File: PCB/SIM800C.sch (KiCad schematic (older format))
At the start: 35 parts, among them J10 Conn_01x05, J11 Conn_01x02, J8 Conn_01x05, J9 Conn_01x05, U10 GSM_SMA, U11 BT_SMA, U12 USB_PCB, U3 footprint-lib_nano-sim-card-h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, U4 SMF05C, U5 SIM800C, U6 MIC29302BU

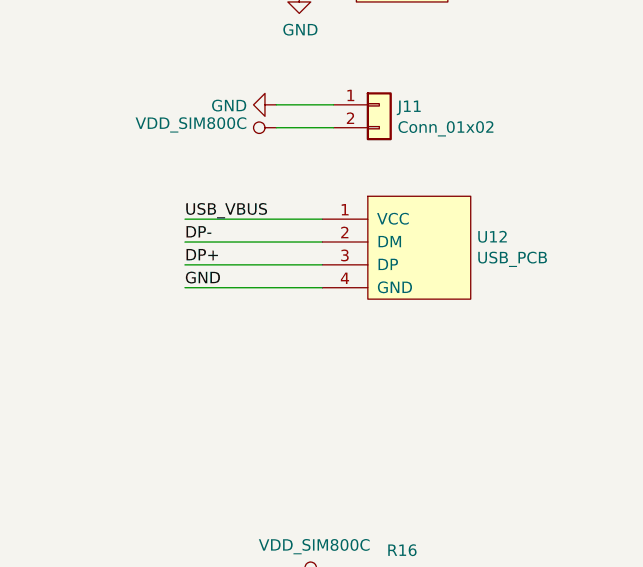
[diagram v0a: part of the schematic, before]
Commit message: updte
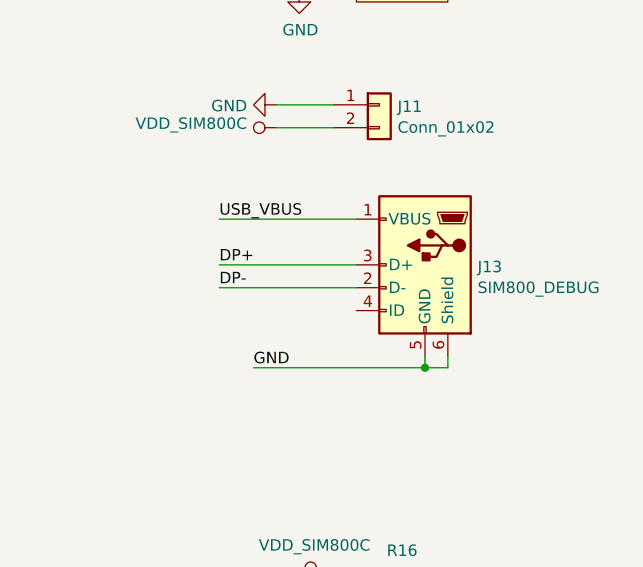
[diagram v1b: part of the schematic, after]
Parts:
- removed U12: USB_PCB, footprint-lib:usb-PCB, symbol taobao-components:USB_PCB
- added J13: SIM800_DEBUG, w_conn_pc:conn_usb_B_micro_smd, symbol Connector:USB_B_Micro
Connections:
- net DP+: now also J13.3 (D+)
- net DP-: now also J13.2 (D-)
- net GND: now also J13.5 (GND), J13.6 (Shield)
- net USB_VBUS: now also J13.1 (VBUS)
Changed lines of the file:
@@
 	15000 8250 15000 8000
 Connection ~ 14550 8250
-$Comp
-L taobao-components:USB_PCB U12
-U 1 1 5BD538D1
-P 14850 6050
-F 0 "U12" H 15177 6121 50  0000 L CNN
-F 1 "USB_PCB" H 15177 6030 50  0000 L CNN
-F 2 "footprint-lib:usb-PCB" H 14850 6100 50  0001 C CNN
-F 3 "" H 14850 6100 50  0001 C CNN
-	1    14850 6050
-	1    0    0    -1
-$EndComp
-Text Label 13900 5900 0    50   ~ 0
+Text Label 14050 5900 0    50   ~ 0
 USB_VBUS
 Wire Wire Line
-	13900 5900 14500 5900
-Text Label 13900 6100 0    50   ~ 0
+	14050 5900 14650 5900
+Text Label 14050 6100 0    50   ~ 0
 DP+
 Wire Wire Line
-	13900 6100 14500 6100
-Text Label 13900 6000 0    50   ~ 0
+	14050 6100 14650 6100
+Text Label 14050 6200 0    50   ~ 0
 DP-
 Wire Wire Line
-	13900 6000 14500 6000
-Text Label 13900 6200 0    50   ~ 0
+	14050 6200 14650 6200
+Text Label 14200 6550 0    50   ~ 0
 GND
-Wire Wire Line
-	13900 6200 14500 6200
 $Comp
 L taobao-tc:TC107,6V C13
@@
 	0    1    1    0
 $EndComp
+$Comp
+L Connector:USB_B_Micro J13
+U 1 1 5BC7E777
+P 14950 6100
+F 0 "J13" H 14720 6091 50  0000 R CNN
+F 1 "SIM800_DEBUG" H 14720 6000 50  0000 R CNN
+F 2 "w_conn_pc:conn_usb_B_micro_smd" H 15100 6050 50  0001 C CNN
+F 3 "~" H 15100 6050 50  0001 C CNN
+	1    14950 6100
+	-1   0    0    -1
+$EndComp
+Wire Wire Line
+	14950 6550 14950 6500
+Wire Wire Line
+	14200 6550 14950 6550
+Wire Wire Line
+	14950 6550 15050 6550
+Wire Wire Line
+	15050 6550 15050 6500
+Connection ~ 14950 6550
 $EndSCHEMATC
